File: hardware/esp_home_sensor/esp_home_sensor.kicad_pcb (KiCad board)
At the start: 4 copper layers, 90 x 25 mm, 97 parts, among them J1 Conn_01x04_MountingPin, J2 Conn_01x04_MountingPin, J3 Conn_01x08_MountingPin, J4 USB_C_Receptacle_USB2.0_16P, SW1 SW_Push, SW2 SW_Push, SW3 SW_Push, U1 BQ25170, U2 BQ2970, U3 IRLHS6276TRPBF, U4 TPS62840, U5 TPS62840, U6 ESP32-C6-MINI-1, U7 BME680, U8 VEML3235, U9 WE-TVS-82400102

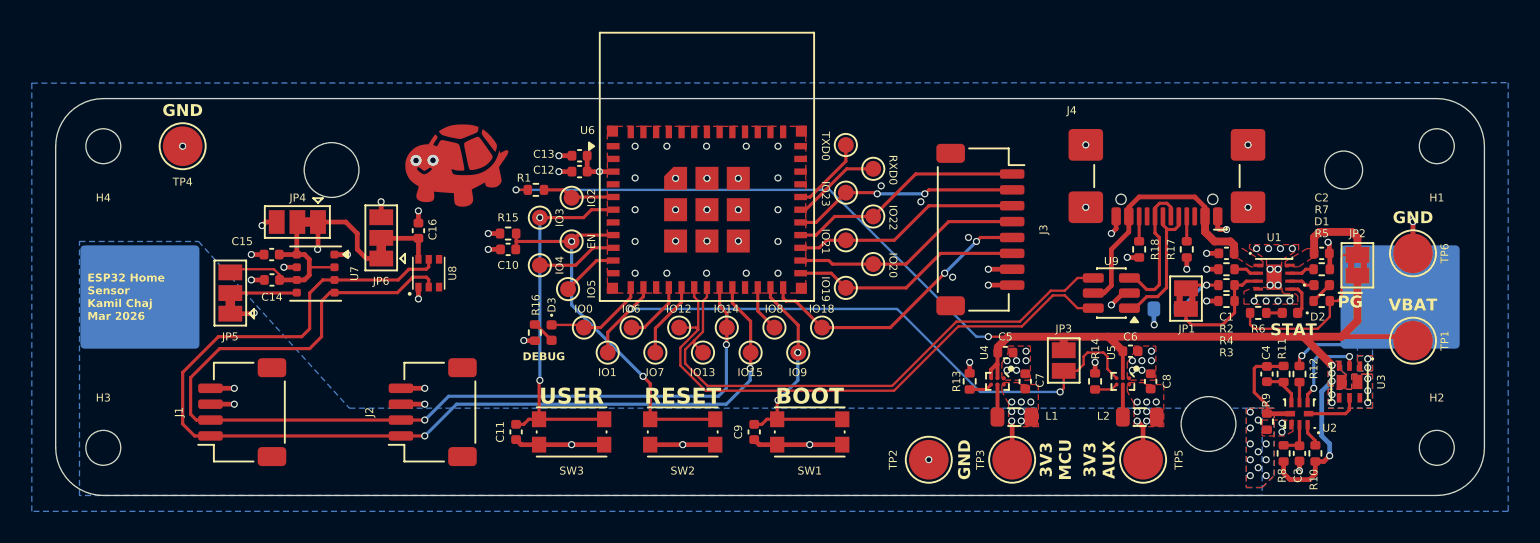
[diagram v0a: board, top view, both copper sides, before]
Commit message: in production
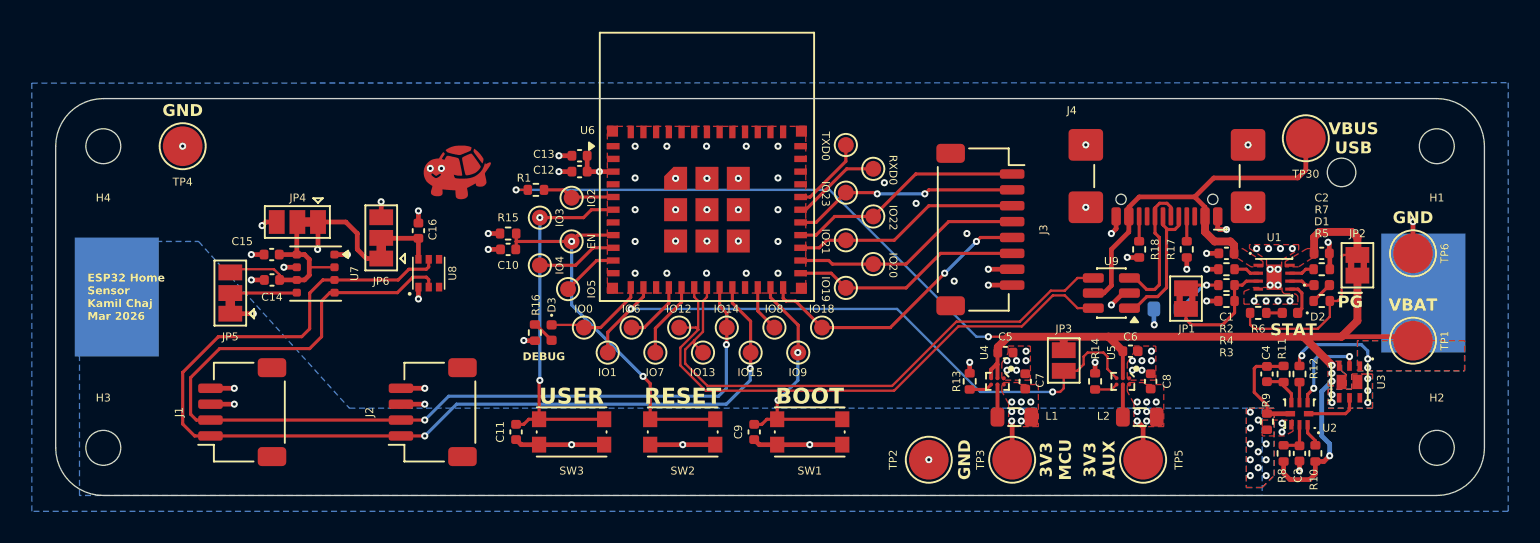
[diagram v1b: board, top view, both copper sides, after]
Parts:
- added TP30: TestPoint, TestPoint:TestPoint_Pad_D2.5mm, F.Cu at (186.2, 53.5)
- BT1: footprint Battery:BatteryHolder_Keystone_1042_1x18650 -> esp_home_sensor:18650_cage
- moved G*** 0.90 mm to (132.8, 55.6)
- turned BT1 to 0 degrees
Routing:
- net /Charger/VIN: track 16.3 -> 26.0 mm
- net /Protection/BAT+: track 8.42 -> 5.92 mm
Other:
- board text added: "VBUS USB"
